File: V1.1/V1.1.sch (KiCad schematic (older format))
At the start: 43 parts, among them SW1 SW_Push, U1 ATmega32U4-AU, U2 SRV05-4, Y1 16MHz

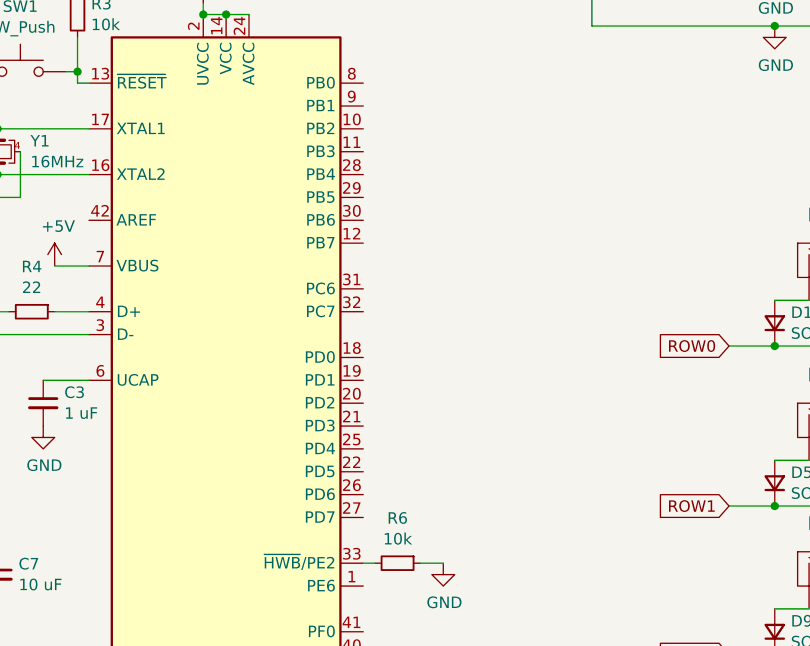
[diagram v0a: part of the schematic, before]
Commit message: PCB and routing done
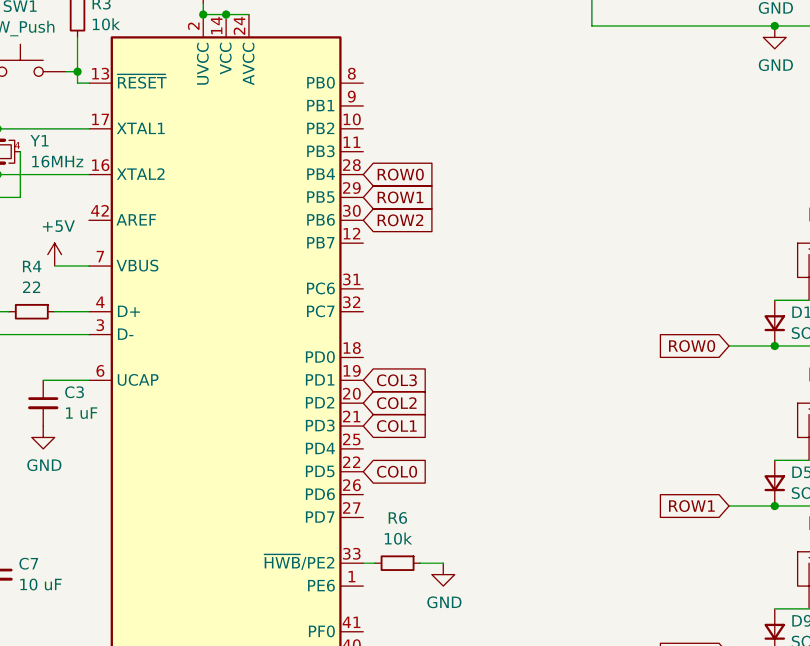
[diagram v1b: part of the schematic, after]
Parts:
- MX1, MX10, MX11, MX12, MX2, MX3, MX4, MX5, MX6, MX7, MX8, MX9: footprint MX_Alps_Hybrid:MX-1U-NoLED -> MX_Only:MXOnly-1U-NoLED
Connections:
- net COL0: now also U1.22 (PD5)
- net COL1: now also U1.21 (PD3)
- net COL2: now also U1.20 (PD2)
- net COL3: now also U1.19 (PD1)
- net ROW0: now also U1.28 (PB4)
- net ROW1: now also U1.29 (PB5)
- net ROW2: now also U1.30 (PB6)
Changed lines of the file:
@@
 F 0 "MX1" H 5483 3673 60  0000 C CNN
 F 1 "MX-NoLED" H 5483 3599 20  0000 C CNN
-F 2 "MX_Alps_Hybrid:MX-1U-NoLED" H 4825 3425 60  0001 C CNN
+F 2 "MX_Only:MXOnly-1U-NoLED" H 4825 3425 60  0001 C CNN
 F 3 "" H 4825 3425 60  0001 C CNN
 	1    5450 3450
@@
 F 0 "MX2" H 6033 3673 60  0000 C CNN
 F 1 "MX-NoLED" H 6033 3599 20  0000 C CNN
-F 2 "MX_Alps_Hybrid:MX-1U-NoLED" H 5375 3425 60  0001 C CNN
+F 2 "MX_Only:MXOnly-1U-NoLED" H 5375 3425 60  0001 C CNN
 F 3 "" H 5375 3425 60  0001 C CNN
 	1    6000 3450
@@
 F 0 "MX3" H 6533 3673 60  0000 C CNN
 F 1 "MX-NoLED" H 6533 3599 20  0000 C CNN
-F 2 "MX_Alps_Hybrid:MX-1U-NoLED" H 5875 3425 60  0001 C CNN
+F 2 "MX_Only:MXOnly-1U-NoLED" H 5875 3425 60  0001 C CNN
 F 3 "" H 5875 3425 60  0001 C CNN
 	1    6500 3450
@@
 F 0 "MX4" H 7083 3673 60  0000 C CNN
 F 1 "MX-NoLED" H 7083 3599 20  0000 C CNN
-F 2 "MX_Alps_Hybrid:MX-1U-NoLED" H 6425 3425 60  0001 C CNN
+F 2 "MX_Only:MXOnly-1U-NoLED" H 6425 3425 60  0001 C CNN
 F 3 "" H 6425 3425 60  0001 C CNN
 	1    7050 3450
@@
 F 0 "MX5" H 5483 4373 60  0000 C CNN
 F 1 "MX-NoLED" H 5483 4299 20  0000 C CNN
-F 2 "MX_Alps_Hybrid:MX-1U-NoLED" H 4825 4125 60  0001 C CNN
+F 2 "MX_Only:MXOnly-1U-NoLED" H 4825 4125 60  0001 C CNN
 F 3 "" H 4825 4125 60  0001 C CNN
 	1    5450 4150
@@
 F 0 "MX6" H 6033 4373 60  0000 C CNN
 F 1 "MX-NoLED" H 6033 4299 20  0000 C CNN
-F 2 "MX_Alps_Hybrid:MX-1U-NoLED" H 5375 4125 60  0001 C CNN
+F 2 "MX_Only:MXOnly-1U-NoLED" H 5375 4125 60  0001 C CNN
 F 3 "" H 5375 4125 60  0001 C CNN
 	1    6000 4150
@@
 F 0 "MX7" H 6533 4373 60  0000 C CNN
 F 1 "MX-NoLED" H 6533 4299 20  0000 C CNN
-F 2 "MX_Alps_Hybrid:MX-1U-NoLED" H 5875 4125 60  0001 C CNN
+F 2 "MX_Only:MXOnly-1U-NoLED" H 5875 4125 60  0001 C CNN
 F 3 "" H 5875 4125 60  0001 C CNN
 	1    6500 4150
@@
 F 0 "MX8" H 7083 4373 60  0000 C CNN
 F 1 "MX-NoLED" H 7083 4299 20  0000 C CNN
-F 2 "MX_Alps_Hybrid:MX-1U-NoLED" H 6425 4125 60  0001 C CNN
+F 2 "MX_Only:MXOnly-1U-NoLED" H 6425 4125 60  0001 C CNN
 F 3 "" H 6425 4125 60  0001 C CNN
 	1    7050 4150
@@
 F 0 "MX9" H 5483 5023 60  0000 C CNN
 F 1 "MX-NoLED" H 5483 4949 20  0000 C CNN
-F 2 "MX_Alps_Hybrid:MX-1U-NoLED" H 4825 4775 60  0001 C CNN
+F 2 "MX_Only:MXOnly-1U-NoLED" H 4825 4775 60  0001 C CNN
 F 3 "" H 4825 4775 60  0001 C CNN
 	1    5450 4800
@@
 F 0 "MX10" H 6033 5023 60  0000 C CNN
 F 1 "MX-NoLED" H 6033 4949 20  0000 C CNN
-F 2 "MX_Alps_Hybrid:MX-1U-NoLED" H 5375 4775 60  0001 C CNN
+F 2 "MX_Only:MXOnly-1U-NoLED" H 5375 4775 60  0001 C CNN
 F 3 "" H 5375 4775 60  0001 C CNN
 	1    6000 4800
@@
 F 0 "MX11" H 6533 5023 60  0000 C CNN
 F 1 "MX-NoLED" H 6533 4949 20  0000 C CNN
-F 2 "MX_Alps_Hybrid:MX-1U-NoLED" H 5875 4775 60  0001 C CNN
+F 2 "MX_Only:MXOnly-1U-NoLED" H 5875 4775 60  0001 C CNN
 F 3 "" H 5875 4775 60  0001 C CNN
 	1    6500 4800
@@
 F 0 "MX12" H 7083 5023 60  0000 C CNN
 F 1 "MX-NoLED" H 7083 4949 20  0000 C CNN
-F 2 "MX_Alps_Hybrid:MX-1U-NoLED" H 6425 4775 60  0001 C CNN
+F 2 "MX_Only:MXOnly-1U-NoLED" H 6425 4775 60  0001 C CNN
 F 3 "" H 6425 4775 60  0001 C CNN
 	1    7050 4800
@@
 Wire Wire Line
 	3700 4750 3800 4750
+Text GLabel 3450 4350 2    50   Input ~ 0
+COL0
+Text GLabel 3450 4150 2    50   Input ~ 0
+COL1
+Text GLabel 3450 4050 2    50   Input ~ 0
+COL2
+Text GLabel 3450 3950 2    50   Input ~ 0
+COL3
+Text GLabel 3450 3050 2    50   Input ~ 0
+ROW0
+Text GLabel 3450 3150 2    50   Input ~ 0
+ROW1
+Text GLabel 3450 3250 2    50   Input ~ 0
+ROW2
 $EndSCHEMATC
